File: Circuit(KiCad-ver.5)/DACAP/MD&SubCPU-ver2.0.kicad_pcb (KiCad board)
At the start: 4 copper layers, 93.1 x 77.7 mm, 88 parts, among them J1 Battery, J10 Raspberry_Pi_2_3, J11 Servo, J12 Motor-ONOFF, J13 Servo-ONOFF, J14 MPU9250, J15 PI-I2C, J16 Motor, J17 USB_B_Micro, J2 ST-I2C, J3 voltmeter, J4 Encoder data, J5 ST-Link, J6 +5V, J7 +5V, J8 3V3, Q1 IPD30N03S2L20ATMA1CT-ND, SW1 CT3073-1-ND, SW2 ST-RST, SW3 PI-RST, U1 VNH5019A, U2 STM32F303K8T6, U3 LM1085IS-5.0/NOPB, U4 LM1085IS-5.0/NOPB

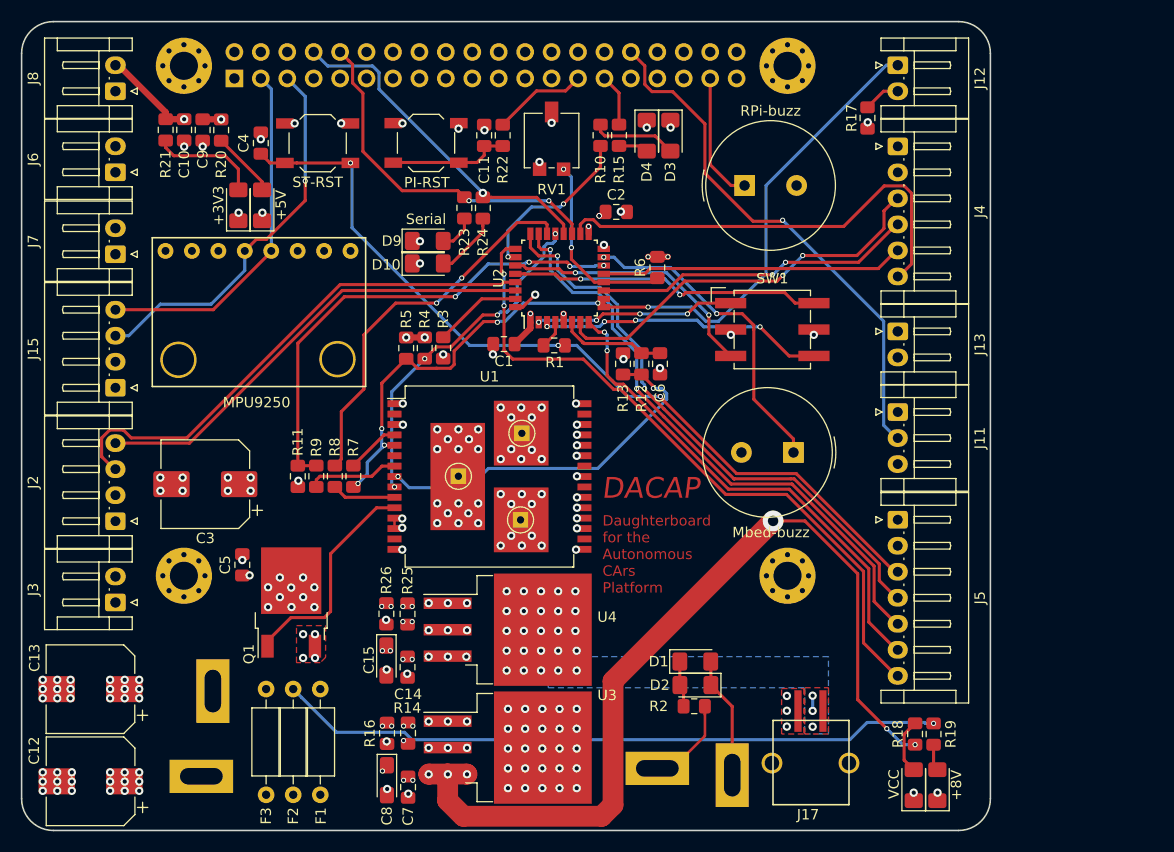
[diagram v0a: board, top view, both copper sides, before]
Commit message: upgrade circuit
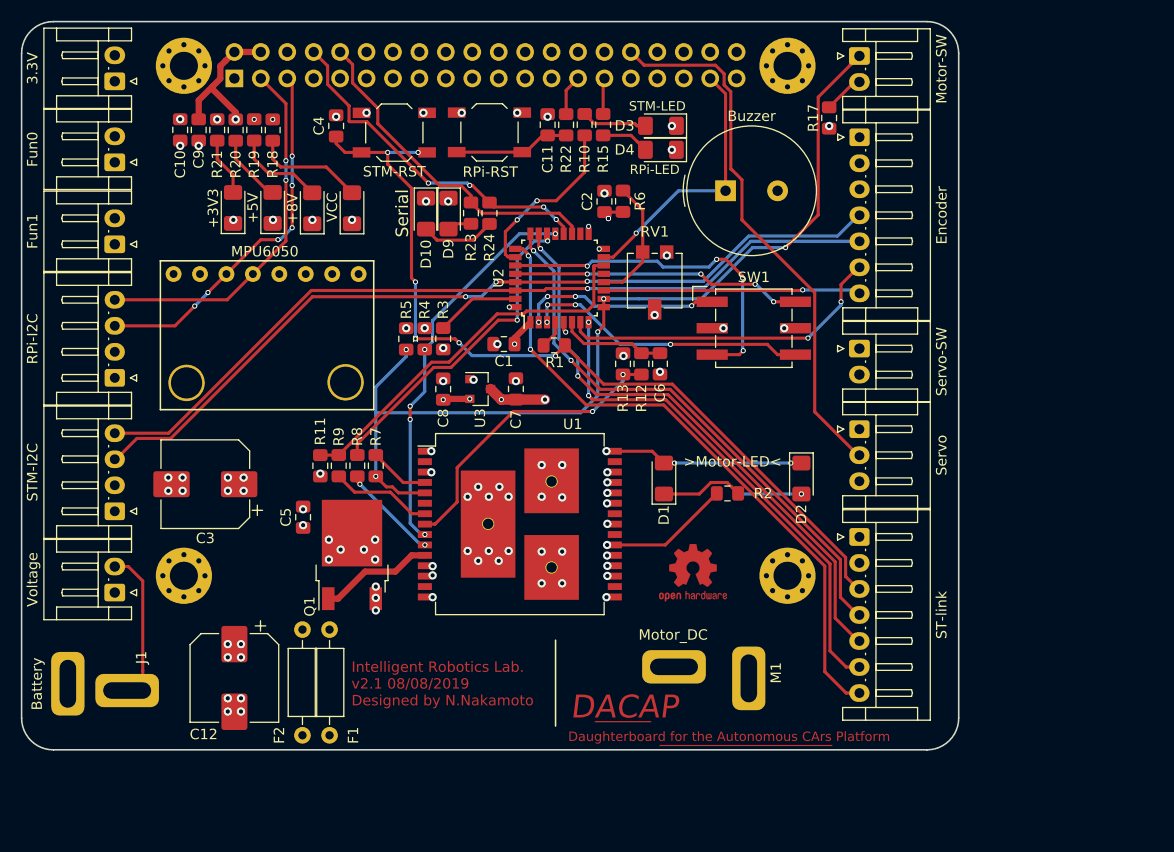
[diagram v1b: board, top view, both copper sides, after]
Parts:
- removed C13: 220uF, Capacitor_SMD:CP_Elec_8x10
- removed C14: 10uF, Capacitor_SMD:C_0805_2012Metric_Pad1.15x1.40mm_HandSolder
- removed C15: tantalum 10uF, Capacitor_Tantalum_SMD:CP_EIA-3216-12_Kemet-S_Pad1.58x1.35mm_HandSolder
- removed F3: Polyfuse, Resistor_THT:R_Axial_DIN0207_L6.3mm_D2.5mm_P10.16mm_Horizontal
- removed J14: MPU9250, self:MPU9250-BMP280
- removed J16: Motor, zisaku:Ultra_male
- removed J17: USB_B_Micro, zisaku:microusbB-supply
- removed J4: Encoder data, Connector_JST:JST_EH_S06B-EH_1x06_P2.50mm_Horizontal
- removed Mbed-buzz: PKM13EPYH4000-A0, Buzzer_Beeper:Buzzer_TDK_PS1240P02BT_D12.2mm_H6.5mm
- removed R14, R25: 121 1%, Resistor_SMD:R_0805_2012Metric_Pad1.15x1.40mm_HandSolder
- removed R16, R26: 365 1%, Resistor_SMD:R_0805_2012Metric_Pad1.15x1.40mm_HandSolder
- removed the REF** at (85.0, 110.1)
- removed the REF** at (91.1, 106.0)
- removed the REF** at (91.0, 114.3)
- removed U4: LM1085IS-5.0/NOPB, Package_TO_SOT_SMD:TO-263-3_TabPin2
- added Encoder: Encoder, Connector_JST:JST_EH_S07B-EH_1x07_P2.50mm_Horizontal, F.Cu at (123.6, 77.5)
- added M1: Motor_DC, zisaku:Ultra_female, B.Cu at (113.5, 131.6)
- added MPU6050: MPU6050, self:MPU9250-BMP280, F.Cu at (56.1, 89.4)
- added REF**: OSHW-Logo2_7.3x6mm_Copper, zisaku:OSHW-Logo2_7.3x6mm_Copper, F.Cu at (107.6, 119.4)
- added REF**: OSHW-Logo2_7.3x6mm_Copper, Symbol:OSHW-Logo2_7.3x6mm_Copper, F.Cu at (107.6, 119.4)
- added REF**: 1pin, md:1pin-hole, F.Cu at (87.9, 114.7)
- added REF**: 1pin, md:1pin-hole, F.Cu at (94.0, 110.6)
- added REF**: 1pin, md:1pin-hole, F.Cu at (94.0, 118.9)
- C7: value 10uF -> 1uF
- C8: value tantalum 10uF -> 1uF; footprint Capacitor_Tantalum_SMD:CP_EIA-3216-12_Kemet-S_Pad1.58x1.35mm_HandSolder -> Capacitor_SMD:C_0805_2012Metric_Pad1.15x1.40mm_HandSolder
- Fun0: renamed from J6; value +5V -> Fun0
- Fun1: renamed from J7; value +5V -> Fun1
- J1: footprint zisaku:Ultra_female -> zisaku:Ultra_male
- SW2: value ST-RST -> STM-RST
- SW3: value PI-RST -> RPi-RST
- U3: value LM1085IS-5.0/NOPB -> MCP1703A-3302_SOT23; footprint Package_TO_SOT_SMD:TO-263-3_TabPin2 -> Package_TO_SOT_SMD:SOT-23
- moved R19 87.4 mm to (65.4, 76.8)
- moved R18 84.7 mm to (67.2, 76.8), turned to 270 degrees
- moved D6 81.7 mm to (71.0, 84.4)
- moved D5 77.4 mm to (74.8, 84.4)
- moved C7 39.6 mm to (90.6, 101.7), turned to 90 degrees
- moved C8 38.0 mm to (83.6, 101.7), turned to 90 degrees
- moved U3 34.6 mm to (87.1, 101.7)
- moved D2 22.3 mm to (118.0, 110.3), turned to 270 degrees
- moved R2 20.7 mm to (110.9, 111.8), turned to 180 degrees
- moved D1 17.8 mm to (104.8, 110.3), turned to 90 degrees
- moved C12 17.0 mm to (63.5, 129.5), turned to 270 degrees
- moved RV1 16.7 mm to (103.9, 91.3), turned to 90 degrees
- moved J1 16.2 mm to (46.9, 128.0), turned to 270 degrees
- moved SW2 7.44 mm to (78.9, 77.1)
- moved C4 7.42 mm to (73.3, 76.4)
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- renumbered J8 to 3.3V, RPi-buzz to Buzzer, J12 to Motor-SW, J15 to RPi-I2C, J5 to ST-link, J2 to STM-I2C, J11 to Servo, J13 to Servo-SW, J3 to Voltage
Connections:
- C8 pad 1: +5V -> +3V3
- U2 pad 11: Encoder1 -> EncoderB
- U2 pad 13: Encoder2 -> Net-(U2-Pad13)
- U2 pad 15: Net-(LS1-Pad1) -> Net-(J10-Pad37)
- U2 pad 18: Encoder3 -> Net-(U2-Pad18)
- U2 pad 7: Encoder0 -> EncoderA
- U3 pad 1: Net-(R14-Pad2) -> GND
- U3 pad 2: +5V -> +3V3
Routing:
- net VCC: track 107.3 -> 159.2 mm, vias 13 -> 3
- net Encoder3: track 43.7 -> 0.00 mm
- net Encoder0: track 38.3 -> 0.00 mm, vias 2 -> 0
- net ST-SDA: track 44.5 -> 79.2 mm, vias 0 -> 1
- net EncoderA: track 0.00 -> 32.0 mm, vias 0 -> 2
- net ST-SCL: track 50.2 -> 81.9 mm, vias 0 -> 3
- net Net-(LS1-Pad1): track 30.9 -> 0.00 mm, vias 2 -> 0
- net Encoder1: track 30.9 -> 0.00 mm, vias 2 -> 0
- net Encoder2: track 29.2 -> 0.00 mm
- net EncoderB: track 0.00 -> 24.7 mm, vias 0 -> 1
- net GND: track 26.2 -> 4.32 mm, vias 67 -> 47
- net Vout: track 22.8 -> 2.26 mm, vias 35 -> 25
- net +8V: track 66.6 -> 50.0 mm, vias 5 -> 4
- net Net-(J10-Pad37): track 12.4 -> 25.8 mm, vias 0 -> 1
- net Net-(Q1-Pad1): track 21.3 -> 11.0 mm
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- removed copper zone on B.Cu, net +5V
- removed copper zone on F.Cu, net +5V
- removed copper zone on In1.Cu, net +5V
- removed copper zone on F.Cu, net +8V
- removed copper zone on F.Cu, net GND
- removed copper zone on In1.Cu, net Net-(R14-Pad2)
- removed copper zone on In1.Cu, net Net-(R25-Pad2)
- removed copper zone on In1.Cu, net VCC
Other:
- board size 93.1 x 77.7 mm -> 90 x 70 mm
- rule trace_min: 0.2 -> 0.1
- board text added: "-"
- board text added: ">Motor-LED<"
- board text added: "Intelligent Robotics Lab. v2.1 08/08/2019 Designed by N.Nakamoto"
- board text added: "RPi-LED"
- board text added: "STM-LED"
